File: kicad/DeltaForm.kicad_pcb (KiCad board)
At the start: 2 copper layers, 85.4 x 128.6 mm, 66 parts

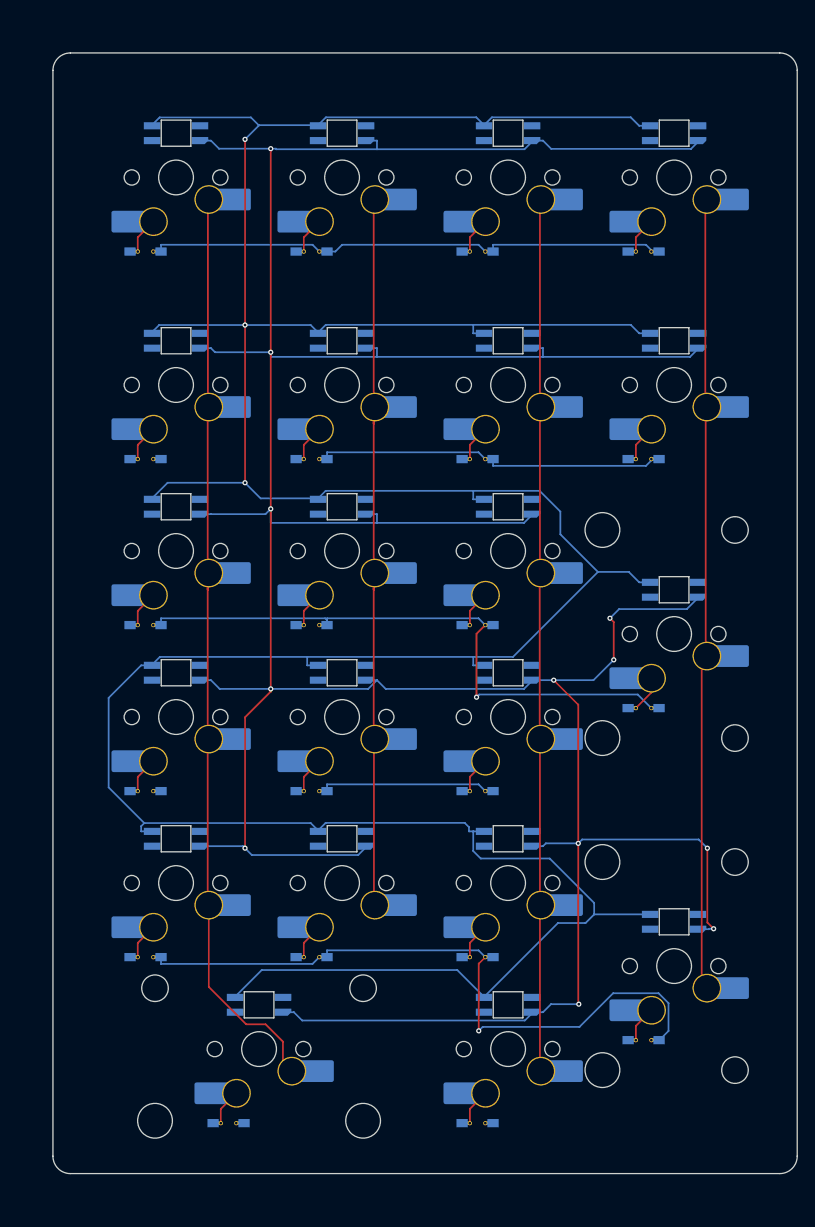
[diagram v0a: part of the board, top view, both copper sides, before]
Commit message: updated MCU
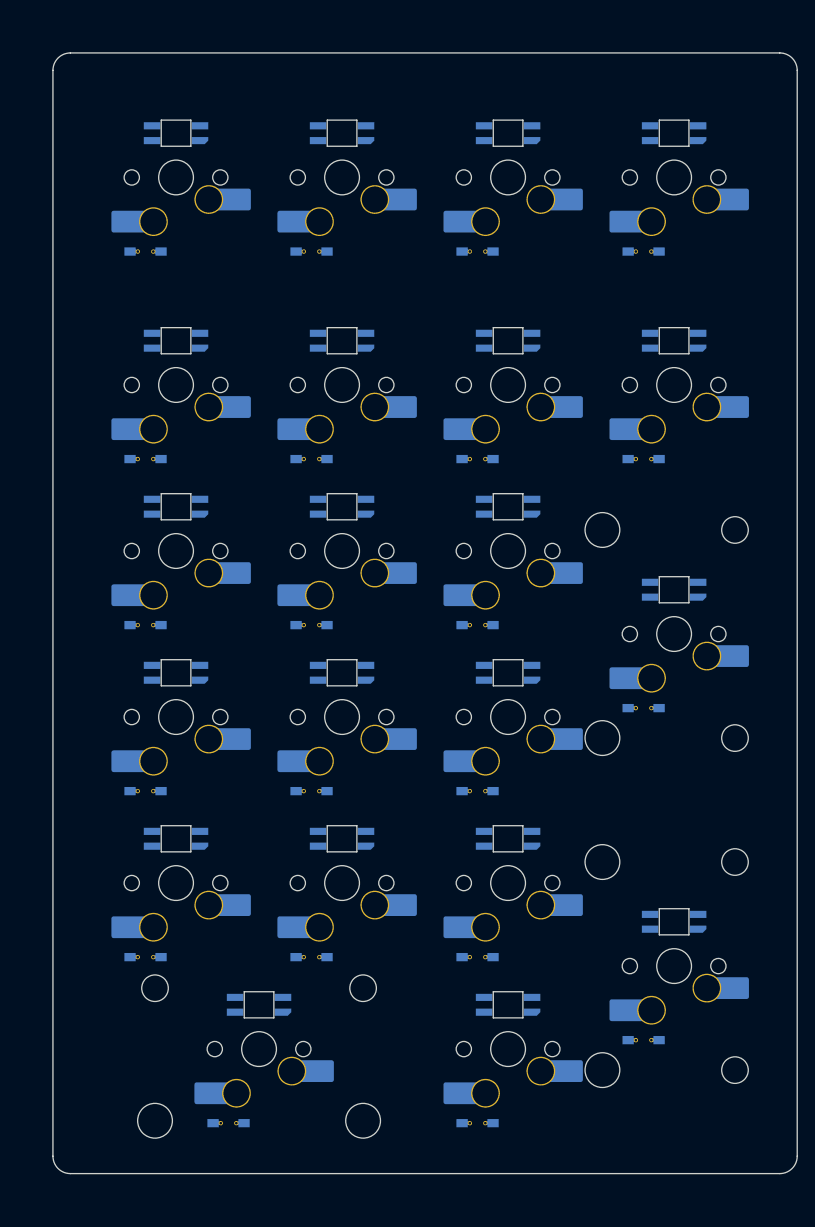
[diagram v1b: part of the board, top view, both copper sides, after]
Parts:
- D1, D10, D11, D12, D13, D14, D15, D16, D17, D18, D19, D2, D20, D21, D3, D4, D5, D6, D7, D8, D9: value 1N4148W -> (none)
- S1, S10, S11, S12, S13, S14, S15, S16, S17, S18, S19, S2, S20, S3, S4, S5, S6, S7, S8, S9: value SW_MX_HS -> (none)
- S21: value SW_MX_HS -> (none); footprint TB2086_KEYSWITCH:SW_MX_HS_2u -> TB2086_KEYSWITCH:SW_MX_HS_1u
- STB1, STB2, STB3: value MX_stab -> Stabilizer_Cherry_MX_2.00u
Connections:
- net Net-(D1-A) renamed c17_func
- net Net-(D10-A) renamed c18_top
- net Net-(D11-A) renamed c19_top
- net Net-(D12-A) renamed c17_home
- net Net-(D13-A) renamed c18_home
- net Net-(D14-A) renamed c19_home
- net Net-(D15-A) renamed c17_bottom
- net Net-(D16-A) renamed c18_bottom
- net Net-(D17-A) renamed c19_bottom
- net Net-(D18-A) renamed c18_thumb
- net Net-(D19-A) renamed c20_top
- net Net-(D2-A) renamed c17_number
- net Net-(D20-A) renamed c20_bottom
- net Net-(D21-A) renamed c17_thumb
- net Net-(D3-A) renamed c18_func
- net Net-(D4-A) renamed c18_number
- net Net-(D5-A) renamed c19_func
- net Net-(D6-A) renamed c19_number
- net Net-(D7-A) renamed c20_func
- net Net-(D8-A) renamed c20_number
- net Net-(D9-A) renamed c17_top
- net row_12 renamed function
- net row_13 renamed number
- net row_14 renamed top
- net row_15 renamed home
- net row_16 renamed bottom
- net row_17 renamed thumb
- S1 pad 2: col_3 -> col_1
- S10 pad 2: col_4 -> col_1
- S11 pad 2: col_5 -> col_4
- S12 pad 2: col_3 -> col_1
- S13 pad 2: col_4 -> col_1
- S14 pad 2: col_5 -> col_4
- S15 pad 2: col_3 -> col_1
- S16 pad 2: col_4 -> col_1
- S17 pad 2: col_5 -> col_4
- S18 pad 2: col_5 -> col_1
- S19 pad 2: col_6 -> col_3
- S2 pad 2: col_3 -> col_1
- S20 pad 2: col_6 -> col_3
- S21 pad 2: col_3 -> col_1
- S3 pad 2: col_4 -> col_1
- S4 pad 2: col_4 -> col_1
- S5 pad 2: col_5 -> col_4
- S6 pad 2: col_5 -> col_4
- S7 pad 2: col_6 -> col_3
- S8 pad 2: col_6 -> col_3
- S9 pad 2: col_3 -> col_1
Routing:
- net GND: track 441.7 -> 0.00 mm, vias 12 -> 0
- net VCC: track 429.4 -> 0.00 mm, vias 3 -> 0
- net col_3: track 123.9 -> 0.00 mm
- net col_5: track 116.8 -> 0.00 mm
- net col_6: track 102.1 -> 0.00 mm
- net col_4: track 98.7 -> 0.00 mm
- net bottom: track 80.2 -> 0.00 mm, vias 1 -> 0
- net top: track 73.5 -> 0.00 mm, vias 1 -> 0
- net function: track 61.0 -> 0.00 mm
- net number: track 42.2 -> 0.00 mm
- net home: track 21.9 -> 0.00 mm
- net c19_top: track 7.79 -> 0.00 mm
- net c19_bottom: track 7.79 -> 0.00 mm
- net c19_number: track 7.79 -> 0.00 mm
- net c19_func: track 7.79 -> 0.00 mm
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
